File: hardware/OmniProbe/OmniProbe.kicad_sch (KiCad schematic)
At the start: 71 parts, among them J1 USB_C_Receptacle_USB2.0_16P, J10 Conn_01x04_Socket, J2 Conn_ARM_JTAG_SWD_10, J3 Conn_01x20_Socket, J4 Conn_01x06_Socket, J5 Conn_ARM_JTAG_SWD_10, J6 Conn_01x03_Socket, J7 Conn_01x03_Socket, J9 Conn_01x04_Socket, U1 RP2040, U2 W25Q128JVP, U3 AP2112K-3.3, U4 TXS0108EPW, U5 TPD2E2U06DCK, U6 SN74LVC8T245, U7 SN74LVC8T245, Y1 12MHz

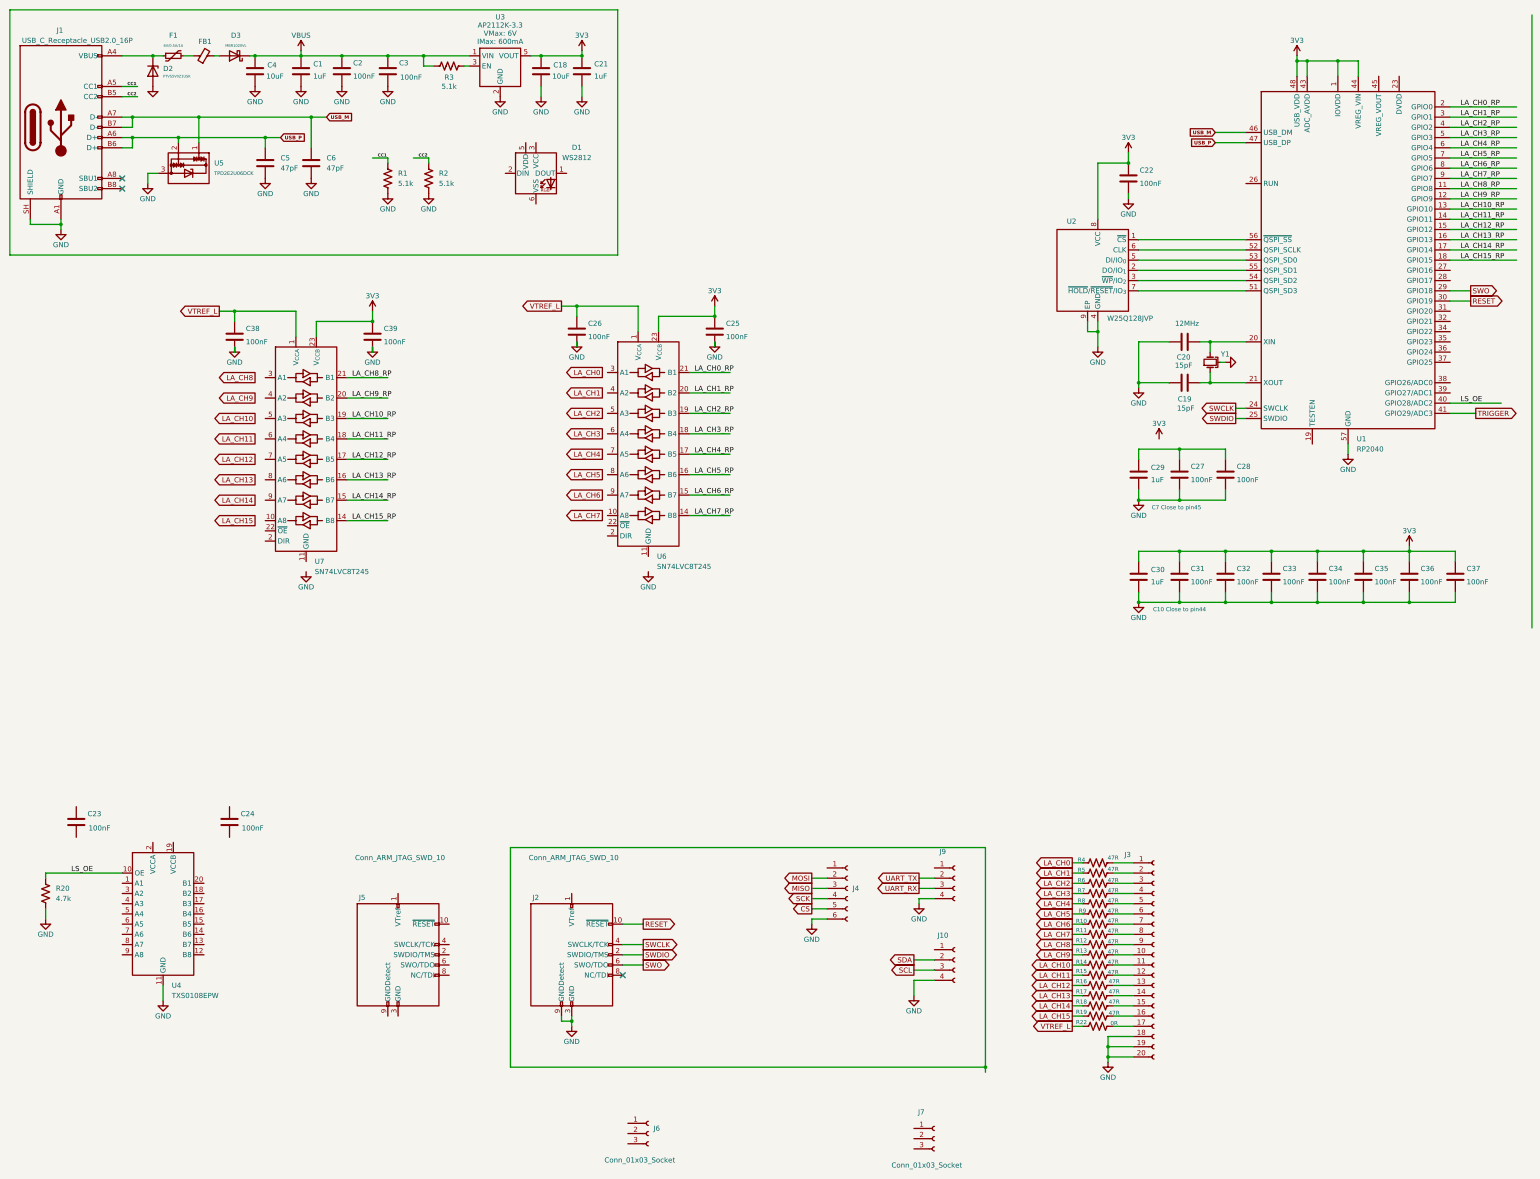
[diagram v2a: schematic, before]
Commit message: v0
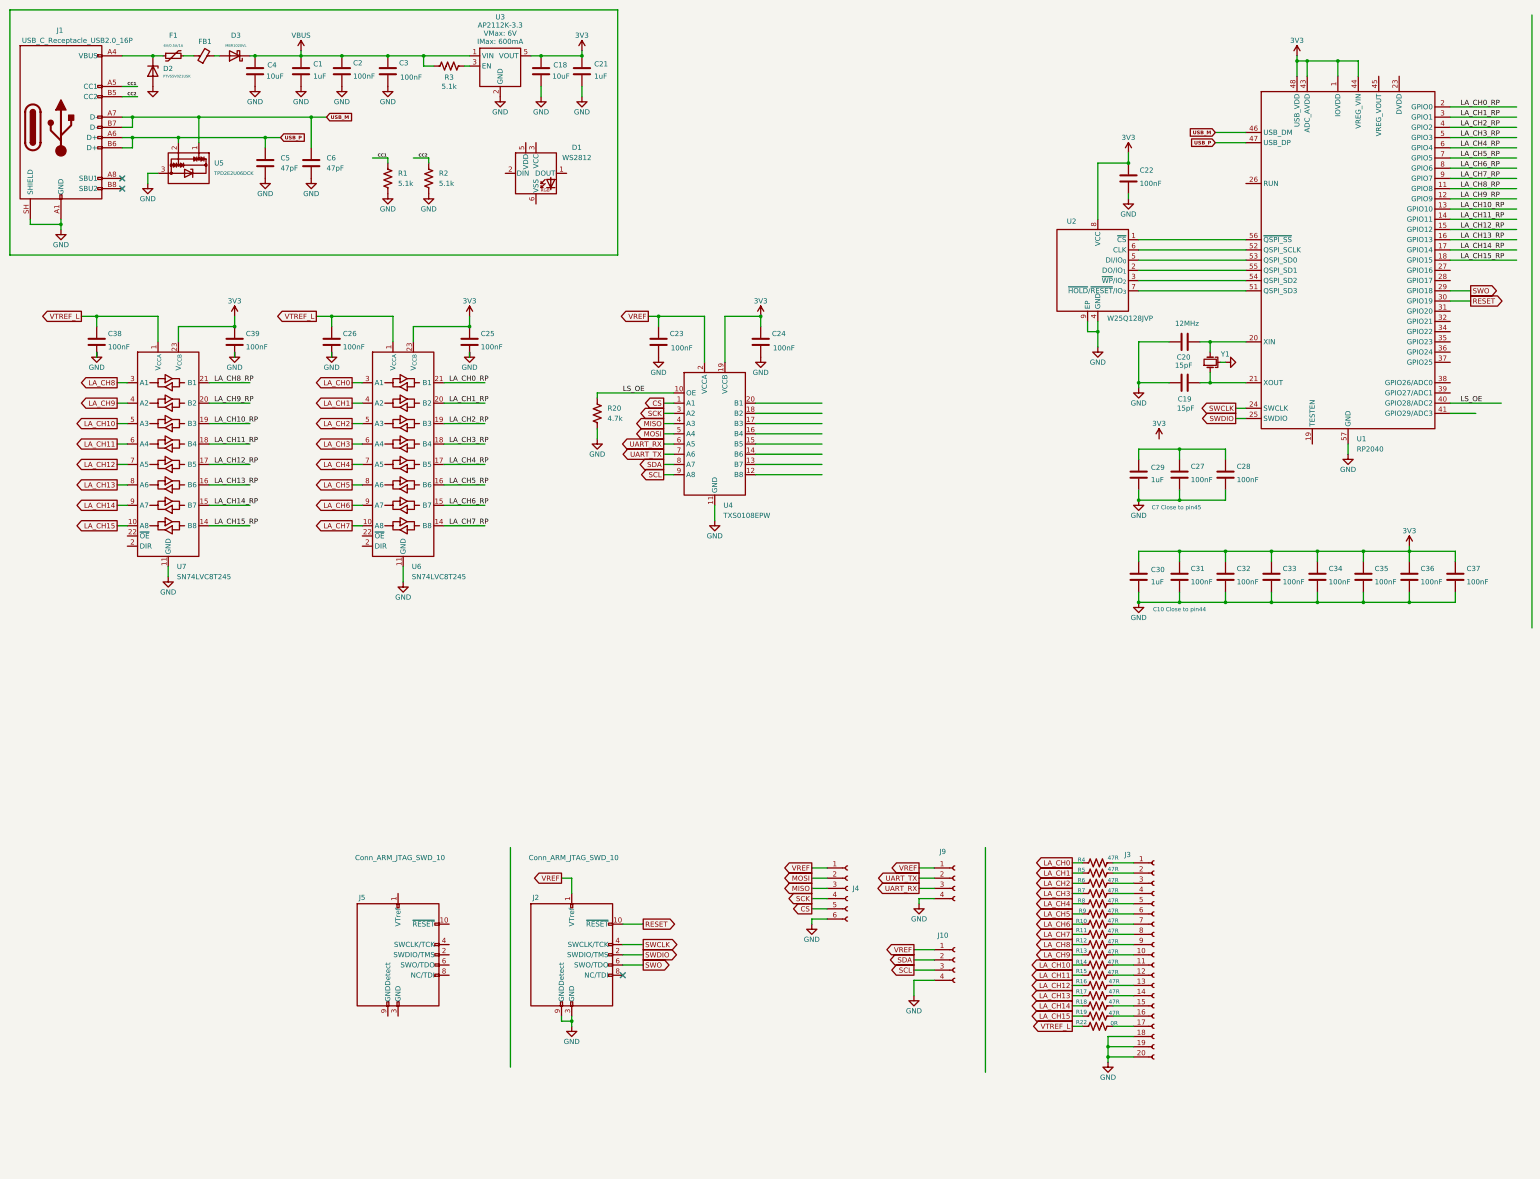
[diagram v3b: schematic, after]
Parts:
- removed J6, J7: Conn_01x03_Socket, Connector_PinHeader_2.54mm:PinHeader_1x03_P2.54mm_Vertical, symbol Connector:Conn_01x03_Socket
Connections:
- net 3V3: now also C24.1, U4.19 (VCCB)
- net CS: now also U4.1 (A1)
- net GND: now also C23.2, C24.2, U6.11 (GND), U6.12 (GND), U6.13 (GND), U7.11 (GND), U7.12 (GND), U7.13 (GND)
- net LA_CH0: now also U6.3 (A1)
- net LA_CH1: now also U6.4 (A2)
- net LA_CH10: now also U7.5 (A3)
- net LA_CH11: now also U7.6 (A4)
- net LA_CH12: now also U7.7 (A5)
- net LA_CH13: now also U7.8 (A6)
- net LA_CH14: now also U7.9 (A7)
- net LA_CH15: now also U7.10 (A8)
- net LA_CH2: now also U6.5 (A3)
- net LA_CH3: now also U6.6 (A4)
- net LA_CH4: now also U6.7 (A5)
- net LA_CH5: now also U6.8 (A6)
- net LA_CH6: now also U6.9 (A7)
- net LA_CH7: now also U6.10 (A8)
- net LA_CH8: now also U7.3 (A1)
- net LA_CH9: now also U7.4 (A2)
- net MISO: now also U4.4 (A3)
- net MOSI: now also U4.5 (A4)
- net SCK: now also U4.3 (A2)
- net SCL: now also U4.9 (A8)
- net SDA: now also U4.8 (A7)
- net UART_RX: now also U4.6 (A5)
- net UART_TX: now also U4.7 (A6)
- net VREF: now reaches J10.1 (Pin_1)
- net VREF: now also C23.1, J2.1 (VTref), J4.1 (Pin_1), J9.1 (Pin_1), U4.2 (VCCA)
- net TRIGGER: no longer names the net of U1.41 (GPIO29/ADC3)
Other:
- moved on the sheet: C23, C24, C25, C26, C38, C39, R20, U4, U6, U7
